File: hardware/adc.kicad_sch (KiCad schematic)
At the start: 32 parts, among them J301 031-5640-1010, U301 REF3033AIDBZT, U302 MCP6001T-E/OT, U303 ADC141S626CIMM_NOPB, U304 MCP6001T-E/OT

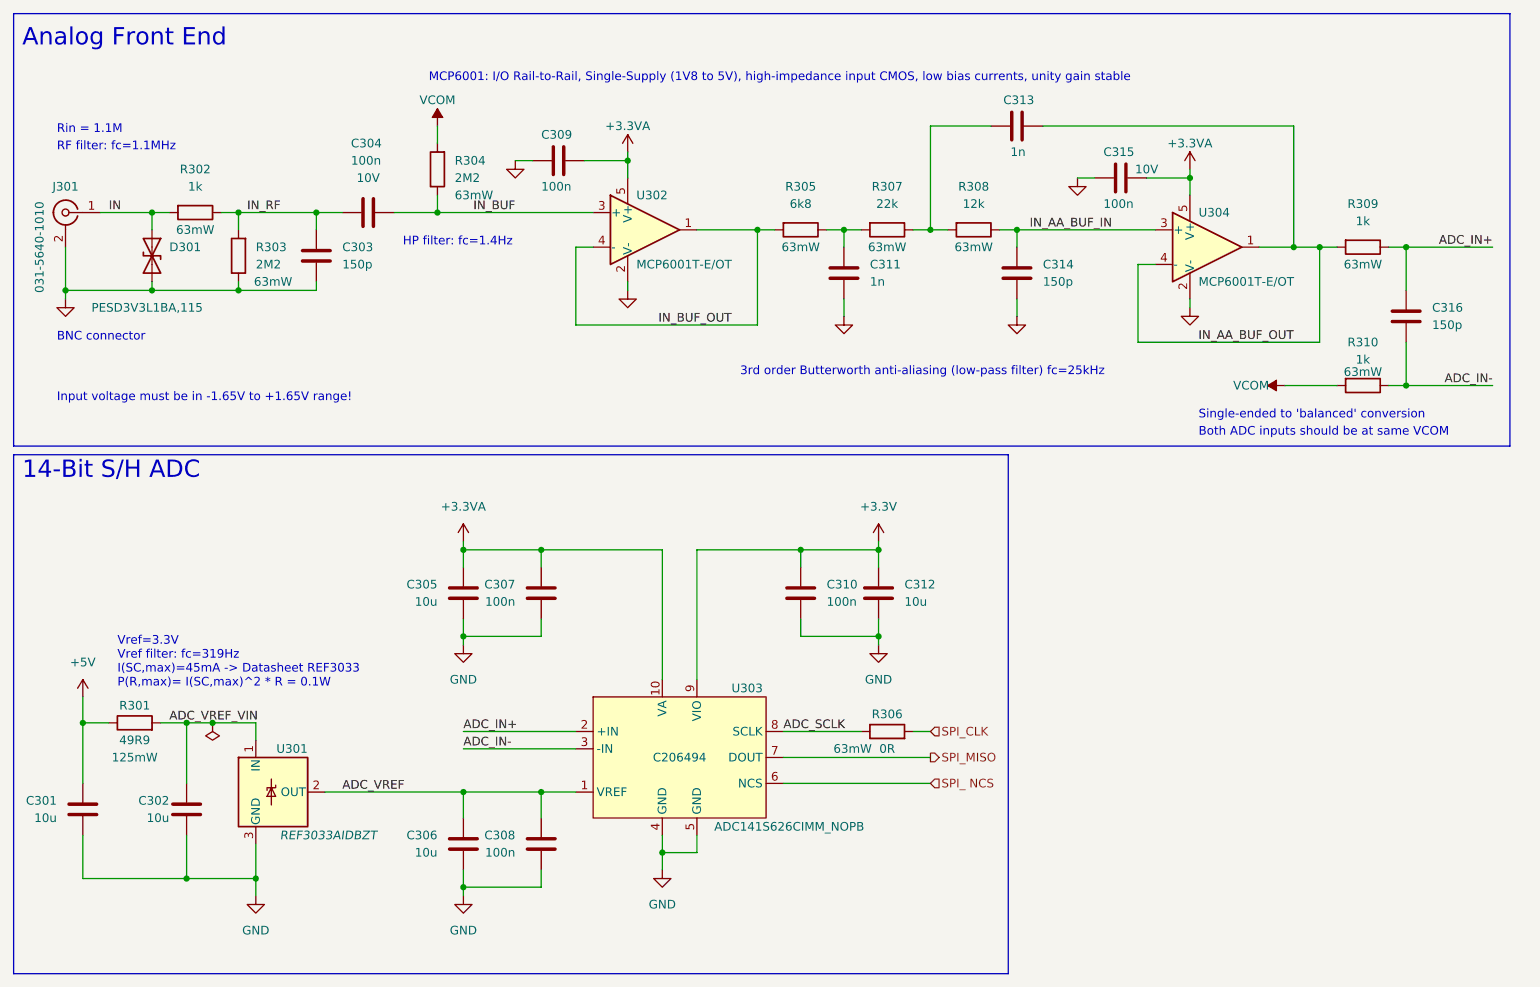
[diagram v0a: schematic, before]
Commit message: Finished routing
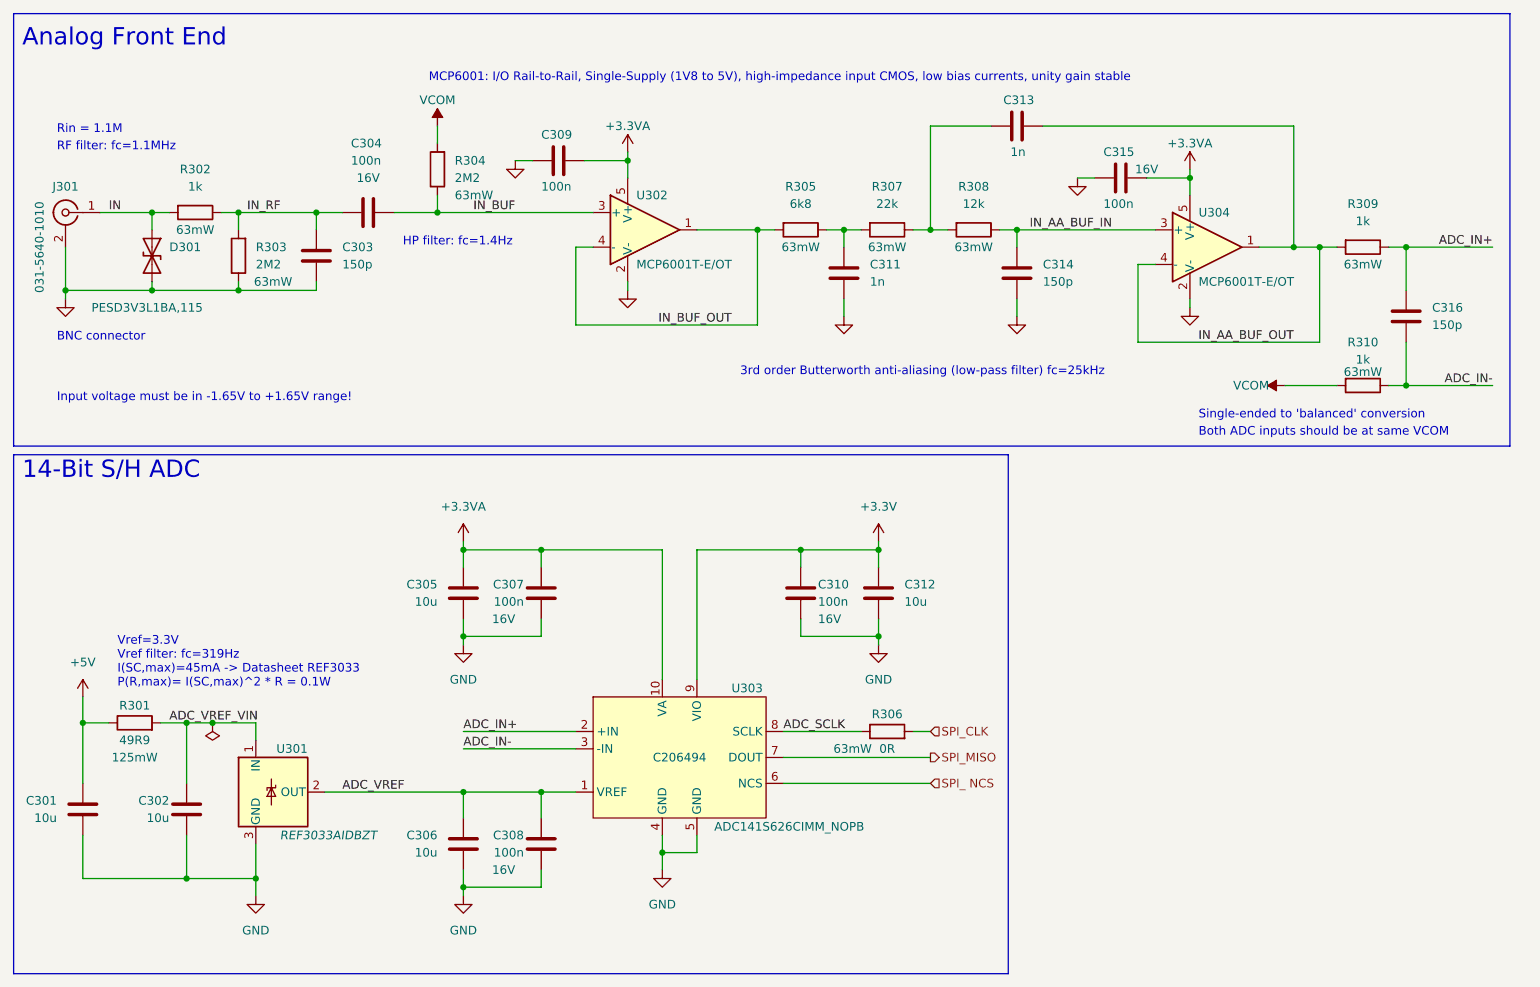
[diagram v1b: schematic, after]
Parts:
- C304, C307, C308, C309, C310, C315: MPN CC0402KRX5R6BB104 -> C1525; Rating 10V -> 16V
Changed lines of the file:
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@@
       (effects (font (size 1.27 1.27)) hide)
     )
-    (property "MPN" "CC0402KRX5R6BB104" (at 71.12 46.99 0)
-      (effects (font (size 1.27 1.27)) hide)
-    )
-    (property "Rating" "10V" (at 71.12 41.91 90)
+    (property "MPN" "C1525" (at 71.12 46.99 0)
+      (effects (font (size 1.27 1.27)) hide)
+    )
+    (property "Rating" "16V" (at 71.12 41.91 90)
       (effects (font (size 1.27 1.27)))
     )
@@
   )
   (symbol (lib_id "Device:C") (at 134.62 102.87 0) (unit 1)
-    (in_bom yes) (on_board yes) (dnp no) (fields_autoplaced)
-    (property "Reference" "C310" (at 138.43 101.5999 0)
-      (effects (font (size 1.27 1.27)) (justify left))
-    )
-    (property "Value" "100n" (at 138.43 104.1399 0)
+    (in_bom yes) (on_board yes) (dnp no)
+    (property "Reference" "C310" (at 137.16 101.6 0)
+      (effects (font (size 1.27 1.27)) (justify left))
+    )
+    (property "Value" "100n" (at 137.16 104.14 0)
       (effects (font (size 1.27 1.27)) (justify left))
     )
@@
       (effects (font (size 1.27 1.27)) hide)
     )
-    (property "MPN" "CC0402KRX5R6BB104" (at 134.62 102.87 0)
-      (effects (font (size 1.27 1.27)) hide)
-    )
-    (property "Rating" "10V" (at 134.62 102.87 0)
-      (effects (font (size 1.27 1.27)) hide)
+    (property "MPN" "C1525" (at 134.62 102.87 0)
+      (effects (font (size 1.27 1.27)) hide)
+    )
+    (property "Rating" "16V" (at 137.16 106.6801 0)
+      (effects (font (size 1.27 1.27)) (justify left))
     )
     (pin "1")
@@
       (effects (font (size 1.27 1.27)) hide)
     )
-    (property "MPN" "CC0402KRX5R6BB104" (at 99.06 39.37 0)
-      (effects (font (size 1.27 1.27)) hide)
-    )
-    (property "Rating" "10V" (at 99.06 39.37 0)
+    (property "MPN" "C1525" (at 99.06 39.37 0)
+      (effects (font (size 1.27 1.27)) hide)
+    )
+    (property "Rating" "16V" (at 99.06 39.37 0)
       (effects (font (size 1.27 1.27)) hide)
     )
@@
   )
   (symbol (lib_id "Device:C") (at 96.52 102.87 0) (mirror y) (unit 1)
-    (in_bom yes) (on_board yes) (dnp no) (fields_autoplaced)
-    (property "Reference" "C307" (at 92.71 101.5999 0)
-      (effects (font (size 1.27 1.27)) (justify left))
-    )
-    (property "Value" "100n" (at 92.71 104.1399 0)
+    (in_bom yes) (on_board yes) (dnp no)
+    (property "Reference" "C307" (at 93.98 101.6 0)
+      (effects (font (size 1.27 1.27)) (justify left))
+    )
+    (property "Value" "100n" (at 93.98 104.14 0)
       (effects (font (size 1.27 1.27)) (justify left))
     )
@@
       (effects (font (size 1.27 1.27)) hide)
     )
-    (property "MPN" "CC0402KRX5R6BB104" (at 96.52 102.87 0)
-      (effects (font (size 1.27 1.27)) hide)
-    )
-    (property "Rating" "10V" (at 96.52 102.87 0)
-      (effects (font (size 1.27 1.27)) hide)
+    (property "MPN" "C1525" (at 96.52 102.87 0)
+      (effects (font (size 1.27 1.27)) hide)
+    )
+    (property "Rating" "16V" (at 92.71 106.6801 0)
+      (effects (font (size 1.27 1.27)) (justify left))
     )
     (pin "1")
@@
     (property "Rating" "125mW" (at 36.83 127 90)
       (effects (font (size 1.27 1.27)))
+    )
+    (property "MPN" "" (at 36.83 121.92 0)
+      (effects (font (size 1.27 1.27)) hide)
     )
     (pin "1")
@@
   )
   (symbol (lib_id "Device:C") (at 96.52 139.7 0) (mirror y) (unit 1)
-    (in_bom yes) (on_board yes) (dnp no) (fields_autoplaced)
-    (property "Reference" "C308" (at 92.71 138.4299 0)
-      (effects (font (size 1.27 1.27)) (justify left))
-    )
-    (property "Value" "100n" (at 92.71 140.9699 0)
+    (in_bom yes) (on_board yes) (dnp no)
+    (property "Reference" "C308" (at 93.98 138.43 0)
+      (effects (font (size 1.27 1.27)) (justify left))
+    )
+    (property "Value" "100n" (at 93.98 140.97 0)
       (effects (font (size 1.27 1.27)) (justify left))
     )
@@
       (effects (font (size 1.27 1.27)) hide)
     )
-    (property "MPN" "CC0402KRX5R6BB104" (at 96.52 139.7 0)
-      (effects (font (size 1.27 1.27)) hide)
-    )
-    (property "Rating" "10V" (at 96.52 139.7 0)
-      (effects (font (size 1.27 1.27)) hide)
+    (property "MPN" "C1525" (at 96.52 139.7 0)
+      (effects (font (size 1.27 1.27)) hide)
+    )
+    (property "Rating" "16V" (at 92.71 143.5101 0)
+      (effects (font (size 1.27 1.27)) (justify left))
     )
     (pin "1")
@@
       (effects (font (size 1.27 1.27)) hide)
     )
-    (property "MPN" "CC0402KRX5R6BB104" (at 181.61 41.91 0)
-      (effects (font (size 1.27 1.27)) hide)
-    )
-    (property "Rating" "10V" (at 185.42 40.64 90)
-      (effects (font (size 1.27 1.27)))
-    )
+    (property "MPN" "C1525" (at 181.61 41.91 0)
+      (effects (font (size 1.27 1.27)) hide)
+    )
+    (property "Rating" "16V" (at 185.42 40.64 90)
+      (effects (font (size 1.27 1.27)))
+    )
